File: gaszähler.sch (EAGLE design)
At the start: 19 parts, among them IC1 LM358D

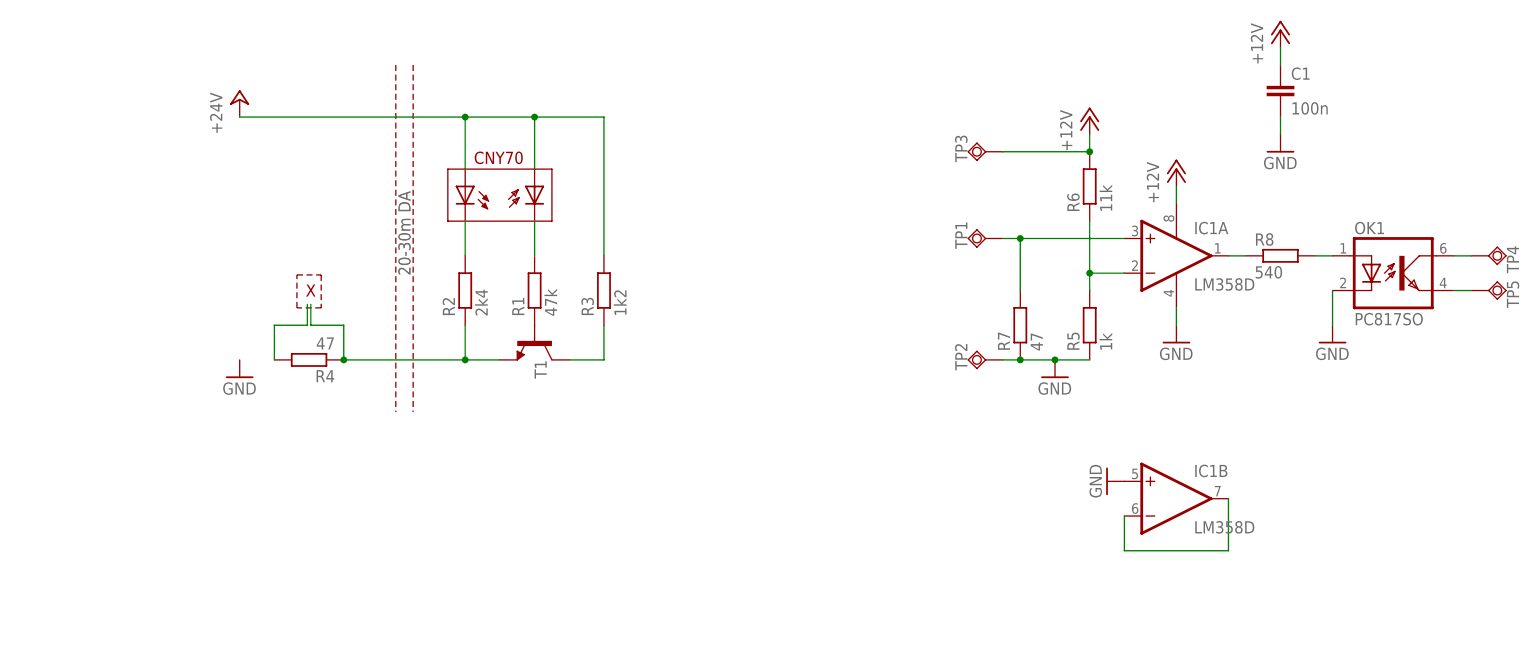
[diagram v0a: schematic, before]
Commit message: adding images
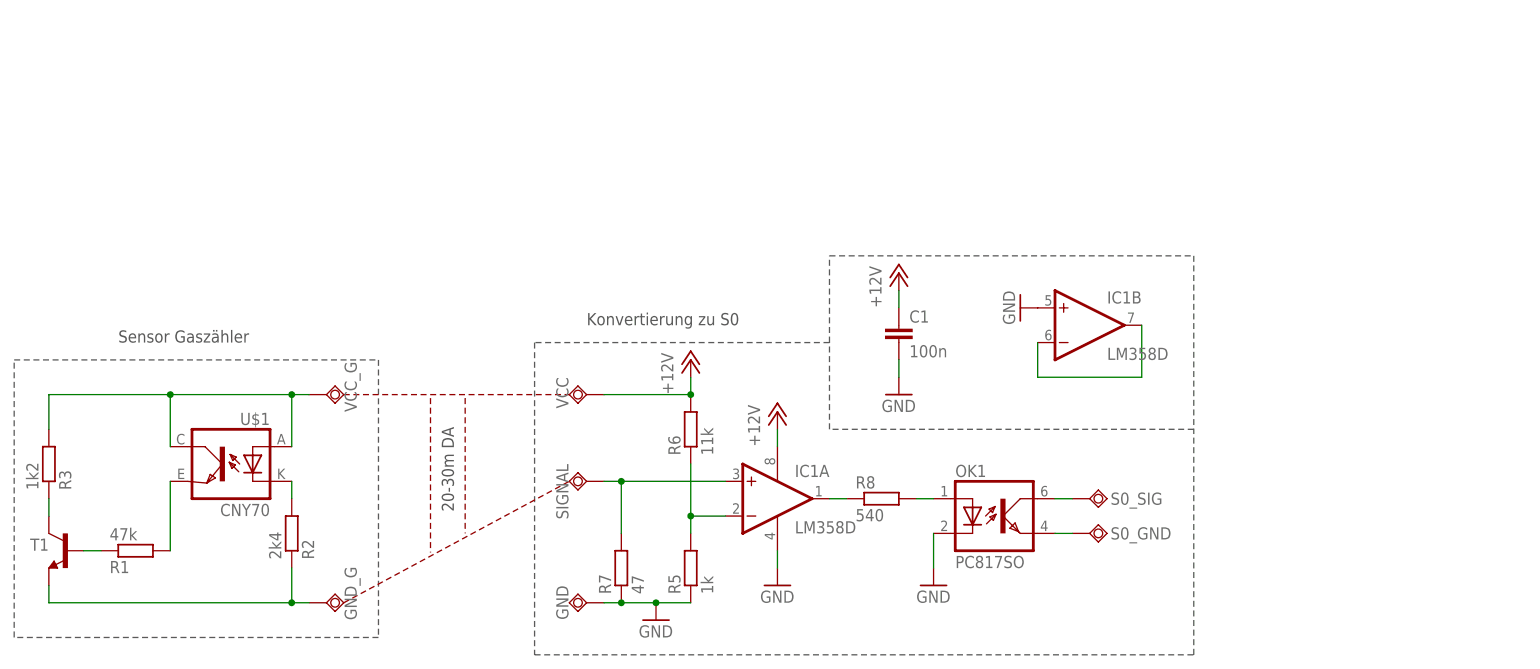
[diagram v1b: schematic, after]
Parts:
- removed D1: BPX65, opto-trans-siemens:BPX65
- removed LED1: (no value), led:LED5MM
- removed R4: 47, rcl:R-EU_0207/10
- removed TP1, TP2, TP3, TP4, TP5: TPSQTP20SQ, testpad:TPSQTP20SQ
- added GND, GND_G, S0_GND, S0_SIG, SIGNAL, VCC, VCC_G: TPSQTP20SQ, testpad:TPSQTP20SQ
- added U$1: CNY70, cny70:CNY70
- R1, R2, R3: device rcl:R-EU_0207/10 -> rcl:R-EU_R0805
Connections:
- removed net +24V: D1.A, LED1.A, R3.2
- removed net N$12: R4.2
- removed net N$4: R2.1, R4.1, T1.E
- new net GND_G: GND_G.TP, R2.1, T1.E
- new net N$14: R3.2, U$1.A, U$1.COL, VCC_G.TP
- net +12V: now also VCC.TP; no longer TP3.TP
- net GND: now also GND.TP; no longer TP2.TP
- net N$10: now also S0_GND.TP; no longer TP5.TP
- net N$2: now also U$1.C; no longer LED1.C
- net N$3: now also U$1.EMI; no longer D1.C
- net N$5: now also SIGNAL.TP; no longer TP1.TP
- net N$8: now also S0_SIG.TP; no longer TP4.TP
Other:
- note added: "Konvertierung zu S0"
- note added: "Sensor Gaszähler"
- note removed: "CNY70"
- note removed: "X"
- moved on the sheet: C1, IC1A, IC1B, OK1, R1, R2, R3, R5, R6, R7, R8, T1
